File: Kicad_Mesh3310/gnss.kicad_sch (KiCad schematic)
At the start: 5 parts, among them U2 NRF9151-LACA-R7

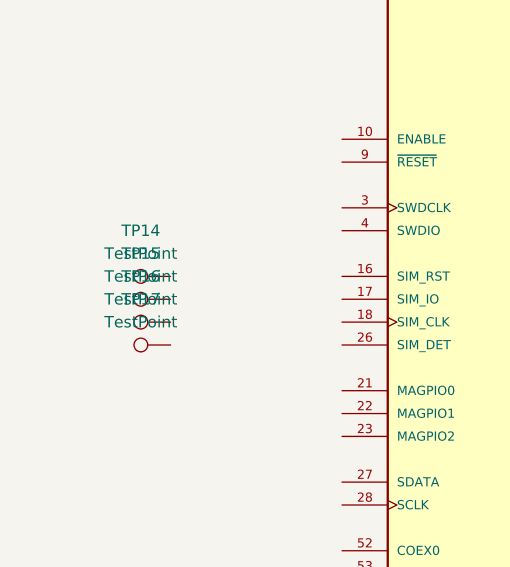
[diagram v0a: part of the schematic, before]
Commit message: Backup work
Adding some extra pads
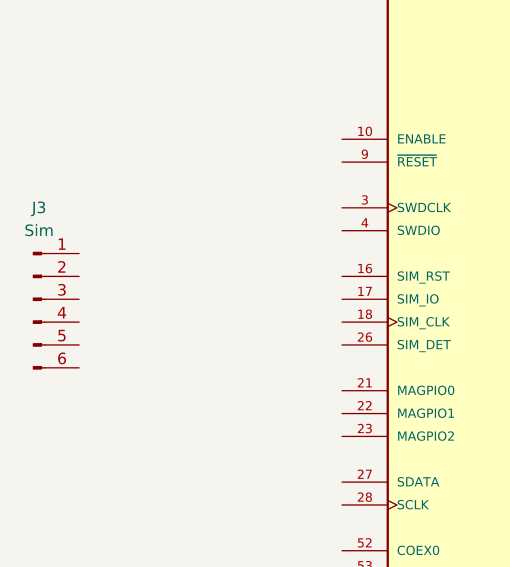
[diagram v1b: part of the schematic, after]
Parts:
- removed TP14, TP15, TP16, TP17: TestPoint, symbol Connector:TestPoint
- added J3: Sim, mesh3310_footprints:3310_sim, symbol Connector:Conn_01x06_Pin
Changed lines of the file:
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@@
-	)
-	(symbol
-		(lib_id "Connector:TestPoint")
-		(at 48.26 86.36 90)
-		(unit 1)
-		(exclude_from_sim no)
-		(in_bom yes)
-		(on_board yes)
-		(dnp no)
-		(fields_autoplaced yes)
-		(property "Reference" "TP17"
-			(at 44.958 81.28 90)
-			(effects
-				(font
-					(size 1.27 1.27)
-				)
-			)
-		)
-		(property "Value" "TestPoint"
-			(at 44.958 83.82 90)
-			(effects
-				(font
-					(size 1.27 1.27)
-				)
-			)
-		)
-		(property "Footprint" ""
-			(at 48.26 81.28 0)
-			(effects
-				(font
-					(size 1.27 1.27)
-				)
-				(hide yes)
-			)
-		)
-		(property "Datasheet" "~"
-			(at 48.26 81.28 0)
-			(effects
-				(font
-					(size 1.27 1.27)
-				)
-				(hide yes)
-			)
-		)
-		(property "Description" "test point"
-			(at 48.26 86.36 0)
-			(effects
-				(font
-					(size 1.27 1.27)
-				)
-				(hide yes)
-			)
-		)
-		(pin "1"
-		)
-		(instances
-			(project "Mesh3310"
-				(path "/8d65c5ef-7a02-4454-aee5-ab9c49e4aeab/98e1aac4-af48-4762-9c2a-9b5d76c64f4f"
-					(reference "TP17")
-					(unit 1)
-				)
-			)
-		)
-	)
-	(symbol
-		(lib_id "Connector:TestPoint")
-		(at 48.26 81.28 90)
-		(unit 1)
-		(exclude_from_sim no)
-		(in_bom yes)
-		(on_board yes)
-		(dnp no)
-		(fields_autoplaced yes)
-		(property "Reference" "TP15"
-			(at 44.958 76.2 90)
-			(effects
-				(font
-					(size 1.27 1.27)
-				)
-			)
-		)
-		(property "Value" "TestPoint"
-			(at 44.958 78.74 90)
-			(effects
-				(font
-					(size 1.27 1.27)
-				)
-			)
-		)
-		(property "Footprint" ""
-			(at 48.26 76.2 0)
-			(effects
-				(font
-					(size 1.27 1.27)
-				)
-				(hide yes)
-			)
-		)
-		(property "Datasheet" "~"
-			(at 48.26 76.2 0)
-			(effects
-				(font
-					(size 1.27 1.27)
-				)
-				(hide yes)
-			)
-		)
-		(property "Description" "test point"
-			(at 48.26 81.28 0)
-			(effects
-				(font
-					(size 1.27 1.27)
-				)
-				(hide yes)
-			)
-		)
-		(pin "1"
-		)
-		(instances
-			(project "Mesh3310"
-				(path "/8d65c5ef-7a02-4454-aee5-ab9c49e4aeab/98e1aac4-af48-4762-9c2a-9b5d76c64f4f"
-					(reference "TP15")
-					(unit 1)
-				)
-			)
-		)
-	)
-	(symbol
-		(lib_id "Connector:TestPoint")
-		(at 48.26 83.82 90)
-		(unit 1)
-		(exclude_from_sim no)
-		(in_bom yes)
-		(on_board yes)
-		(dnp no)
-		(fields_autoplaced yes)
-		(property "Reference" "TP16"
-			(at 44.958 78.74 90)
-			(effects
-				(font
-					(size 1.27 1.27)
-				)
-			)
-		)
-		(property "Value" "TestPoint"
-			(at 44.958 81.28 90)
-			(effects
-				(font
-					(size 1.27 1.27)
-				)
-			)
-		)
-		(property "Footprint" ""
-			(at 48.26 78.74 0)
-			(effects
-				(font
-					(size 1.27 1.27)
-				)
-				(hide yes)
-			)
-		)
-		(property "Datasheet" "~"
-			(at 48.26 78.74 0)
-			(effects
-				(font
-					(size 1.27 1.27)
-				)
-				(hide yes)
-			)
-		)
-		(property "Description" "test point"
-			(at 48.26 83.82 0)
-			(effects
-				(font
-					(size 1.27 1.27)
-				)
-				(hide yes)
-			)
-		)
-		(pin "1"
-		)
-		(instances
-			(project "Mesh3310"
-				(path "/8d65c5ef-7a02-4454-aee5-ab9c49e4aeab/98e1aac4-af48-4762-9c2a-9b5d76c64f4f"
-					(reference "TP16")
-					(unit 1)
-				)
-			)
-		)
-	)
-	(symbol
-		(lib_id "Connector:TestPoint")
-		(at 48.26 78.74 90)
-		(unit 1)
-		(exclude_from_sim no)
-		(in_bom yes)
-		(on_board yes)
-		(dnp no)
-		(fields_autoplaced yes)
-		(property "Reference" "TP14"
-			(at 44.958 73.66 90)
-			(effects
-				(font
-					(size 1.27 1.27)
-				)
-			)
-		)
-		(property "Value" "TestPoint"
-			(at 44.958 76.2 90)
-			(effects
-				(font
-					(size 1.27 1.27)
-				)
-			)
-		)
-		(property "Footprint" ""
-			(at 48.26 73.66 0)
-			(effects
-				(font
-					(size 1.27 1.27)
-				)
-				(hide yes)
-			)
-		)
-		(property "Datasheet" "~"
-			(at 48.26 73.66 0)
-			(effects
-				(font
-					(size 1.27 1.27)
-				)
-				(hide yes)
-			)
-		)
-		(property "Description" "test point"
-			(at 48.26 78.74 0)
-			(effects
-				(font
-					(size 1.27 1.27)
-				)
-				(hide yes)
-			)
-		)
-		(pin "1"
-		)
-		(instances
-			(project "Mesh3310"
-				(path "/8d65c5ef-7a02-4454-aee5-ab9c49e4aeab/98e1aac4-af48-4762-9c2a-9b5d76c64f4f"
-					(reference "TP14")
-					(unit 1)
-				)
-			)
-		)
 	)
 	(symbol
@@
 					(unit 1)
 				)
+			)
+		)
+	)
+	(symbol
+		(lib_id "Connector:Conn_01x06_Pin")
+		(at 33.02 81.28 0)
+		(unit 1)
+		(exclude_from_sim no)
+		(in_bom yes)
+		(on_board yes)
+		(dnp no)
+		(fields_autoplaced yes)
+		(property "Reference" "J3"
+			(at 33.655 71.12 0)
+			(effects
+				(font
+					(size 1.27 1.27)
+				)
+			)
+		)
+		(property "Value" "Sim"
+			(at 33.655 73.66 0)
+			(effects
+				(font
+					(size 1.27 1.27)
+				)
+			)
+		)
+		(property "Footprint" "mesh3310_footprints:3310_sim"
+			(at 33.02 81.28 0)
+			(effects
+				(font
+					(size 1.27 1.27)
+				)
+				(hide yes)
+			)
+		)
+		(property "Datasheet" "~"
+			(at 33.02 81.28 0)
+			(effects
+				(font
+					(size 1.27 1.27)
+				)
+				(hide yes)
+			)
+		)
+		(property "Description" "Generic connector, single row, 01x06, script generated"
+			(at 33.02 81.28 0)
+			(effects
+				(font
+					(size 1.27 1.27)
+				)
+				(hide yes)
+			)
+		)
+		(pin "5"
+		)
+		(pin "4"
+		)
+		(pin "3"
+		)
+		(pin "1"
+		)
+		(pin "6"
+		)
+		(pin "2"
+		)
+		(instances
+			(project "Mesh3310"
+				(path "/8d65c5ef-7a02-4454-aee5-ab9c49e4aeab/98e1aac4-af48-4762-9c2a-9b5d76c64f4f"
+					(reference "J3")
+					(unit 1)
+				)
